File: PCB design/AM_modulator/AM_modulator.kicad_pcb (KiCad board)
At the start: 2 copper layers, 64.3 x 95.7 mm, 11 parts, among them Q1 MMBT3904

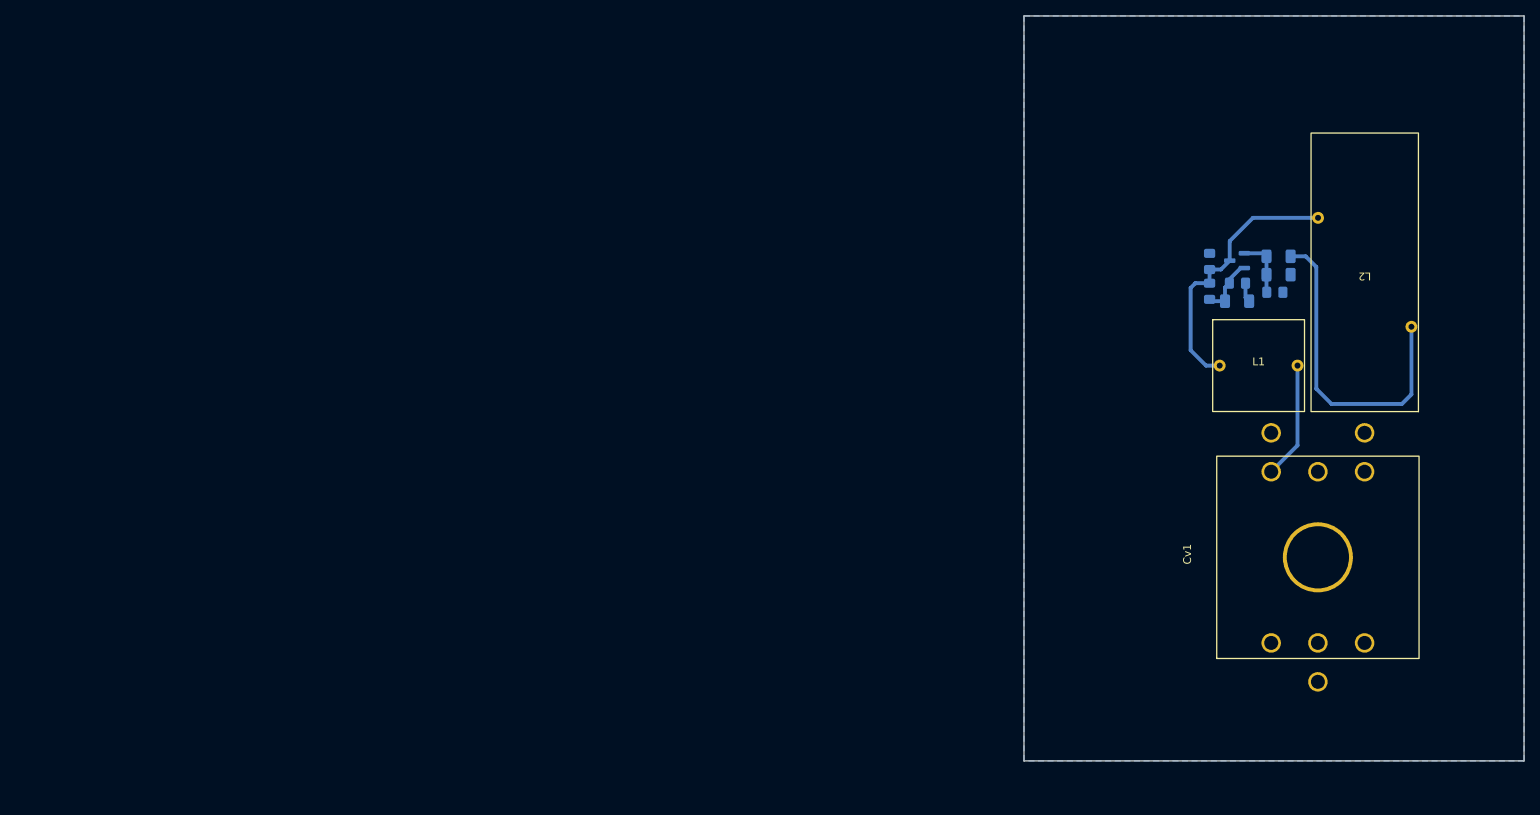
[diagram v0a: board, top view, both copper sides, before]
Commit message: Avances placa
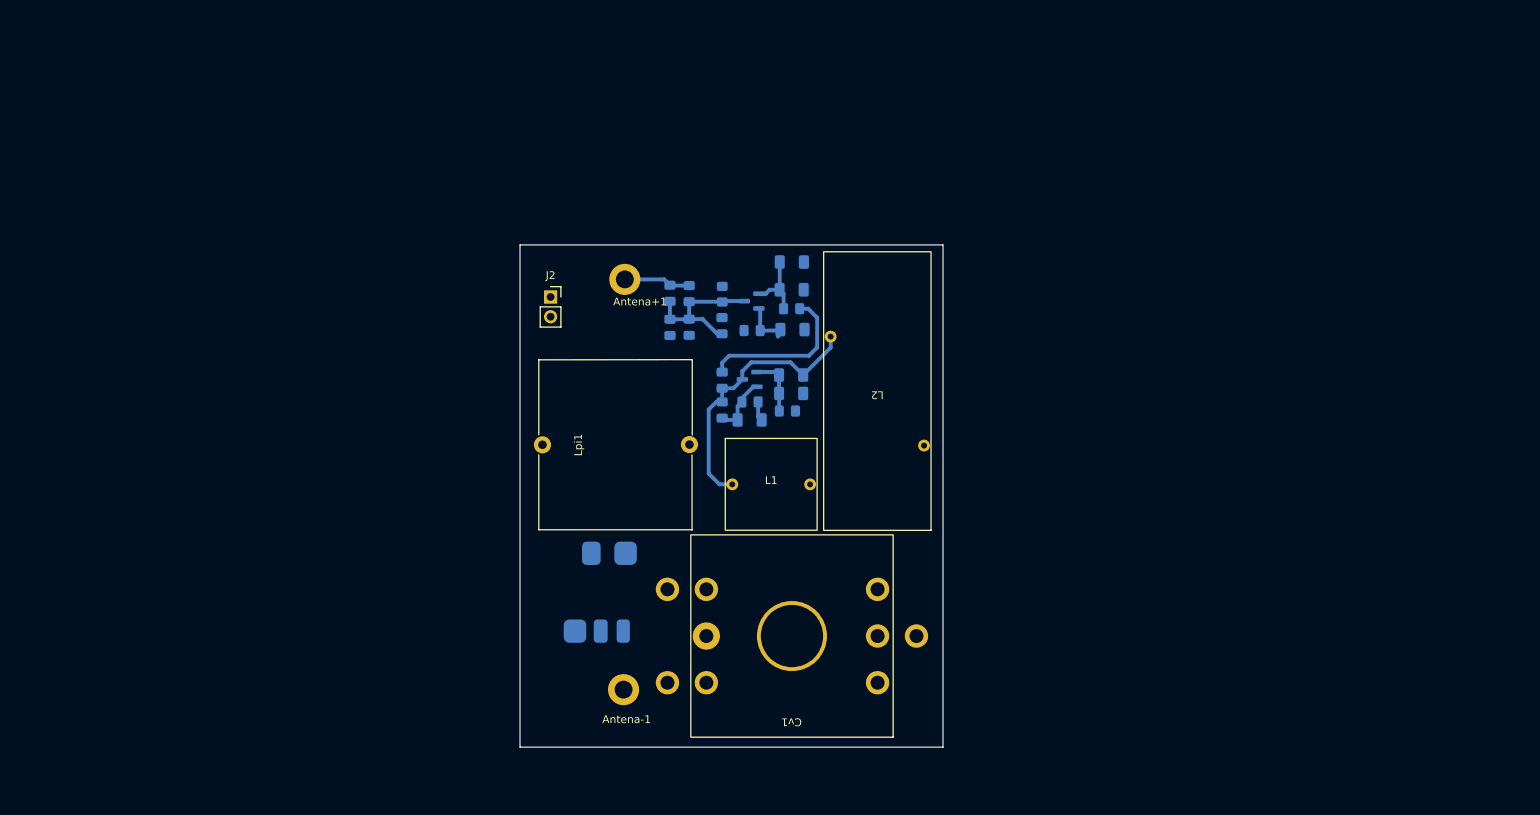
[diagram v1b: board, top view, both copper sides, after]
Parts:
- added Antena+1: Conn_01x01_Female, Connector_Pin:Pin_D1.4mm_L8.5mm_W2.8mm_FlatFork, F.Cu at (120.5, 63.7)
- added Antena-1: Conn_01x01_Female, Connector_Pin:Pin_D1.4mm_L8.5mm_W2.8mm_FlatFork, F.Cu at (120.3, 116.4)
- added CMLO1: 100n, Capacitor_SMD:C_0805_2012Metric_Pad1.18x1.45mm_HandSolder, B.Cu at (141.9, 67.5)
- added CMa1: 100n, Capacitor_SMD:C_0805_2012Metric_Pad1.18x1.45mm_HandSolder, B.Cu at (136.8, 70.3)
- added CMan1: 33p, Capacitor_SMD:C_0805_2012Metric_Pad1.18x1.45mm_HandSolder, B.Cu at (132.9, 69.7)
- added Cpi1: C, Capacitor_SMD:C_0805_2012Metric_Pad1.18x1.45mm_HandSolder, B.Cu at (128.7, 69.8)
- added Cpi11: C, Capacitor_SMD:C_0805_2012Metric_Pad1.18x1.45mm_HandSolder, B.Cu at (126.3, 69.9)
- added Cpi2: C, Capacitor_SMD:C_0805_2012Metric_Pad1.18x1.45mm_HandSolder, B.Cu at (128.7, 65.5)
- added Cpi21: C, Capacitor_SMD:C_0805_2012Metric_Pad1.18x1.45mm_HandSolder, B.Cu at (126.3, 65.5)
- added J1: AudioJack3, Jack Sigma:Jack_Sigma, B.Cu at (117.4, 103.9)
- added J2: Conn_01x02_Female, Connector_PinSocket_2.54mm:PinSocket_1x02_P2.54mm_Vertical, F.Cu at (110.9, 66.0)
- added Lpi1: L, Inductor_THT:L_Toroid_Vertical_L21.6mm_W9.1mm_P8.40mm_Bourns_5700, F.Cu at (109.9, 85.0)
- added QM1: MMBT3904, Package_TO_SOT_SMD:SOT-23, B.Cu at (136.8, 66.5)
- added RMb1: 100k, Resistor_SMD:R_1206_3216Metric_Pad1.30x1.75mm_HandSolder, B.Cu at (141.9, 65.0)
- added RMb2: 100k, Resistor_SMD:R_1206_3216Metric_Pad1.30x1.75mm_HandSolder, B.Cu at (141.9, 61.5)
- added RMc1: 220, Resistor_SMD:R_0805_2012Metric_Pad1.20x1.40mm_HandSolder, B.Cu at (133.0, 65.6)
- added RMe1: 100, Resistor_SMD:R_1206_3216Metric_Pad1.30x1.75mm_HandSolder, B.Cu at (142.0, 70.2)
- moved Cv1 68.3 mm to (141.9, 109.5), turned to 180 degrees
- moved C1 64.5 mm to (133.0, 80.5)
- moved C2 64.5 mm to (136.6, 79.4)
- moved C3 64.5 mm to (141.4, 80.6)
- moved C4 64.5 mm to (133.0, 76.7)
- moved L1 64.5 mm to (139.3, 90.0)
- moved L2 64.5 mm to (152.9, 78.0)
- moved Q1 64.5 mm to (136.5, 76.6)
- moved R1 64.5 mm to (141.8, 76.0)
- moved R2 64.5 mm to (141.8, 78.4)
- moved R3 64.5 mm to (136.5, 81.8)
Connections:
- C4 pad 2: /clapp_oscillator/Vout_30MHz_50Ohm -> /Mixer/LO
- L2 pad 1: +10V -> +12V
- R1 pad 1: +10V -> Net-(C1-Pad1)
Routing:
- net +10V: track 41.7 -> 0.00 mm
- net /Mixer/LO: track 0.00 -> 20.8 mm
- net /Antenna/RF_Antenna: track 0.00 -> 19.2 mm
- net Net-(Cv1-Pad1): track 15.0 -> 0.00 mm
- net Net-(CMLO1-Pad1): track 0.00 -> 9.09 mm
- net Net-(Antena+1-Pad1): track 0.00 -> 8.60 mm
- net Net-(CMa1-Pad1): track 0.00 -> 5.74 mm
- removed copper zone on B.Cu, net GND
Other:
- board size 64.3 x 95.7 mm -> 54.4 x 64.5 mm

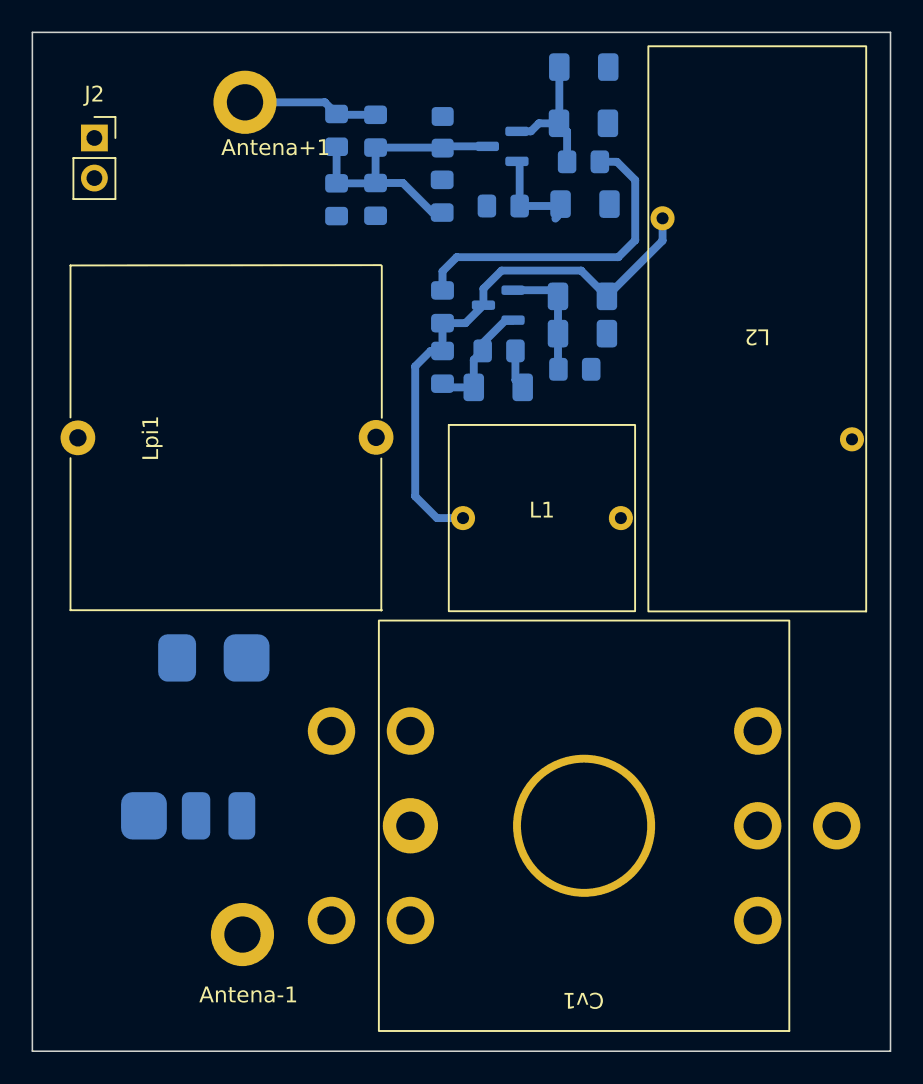
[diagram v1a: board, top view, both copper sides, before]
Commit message: Placa terminada
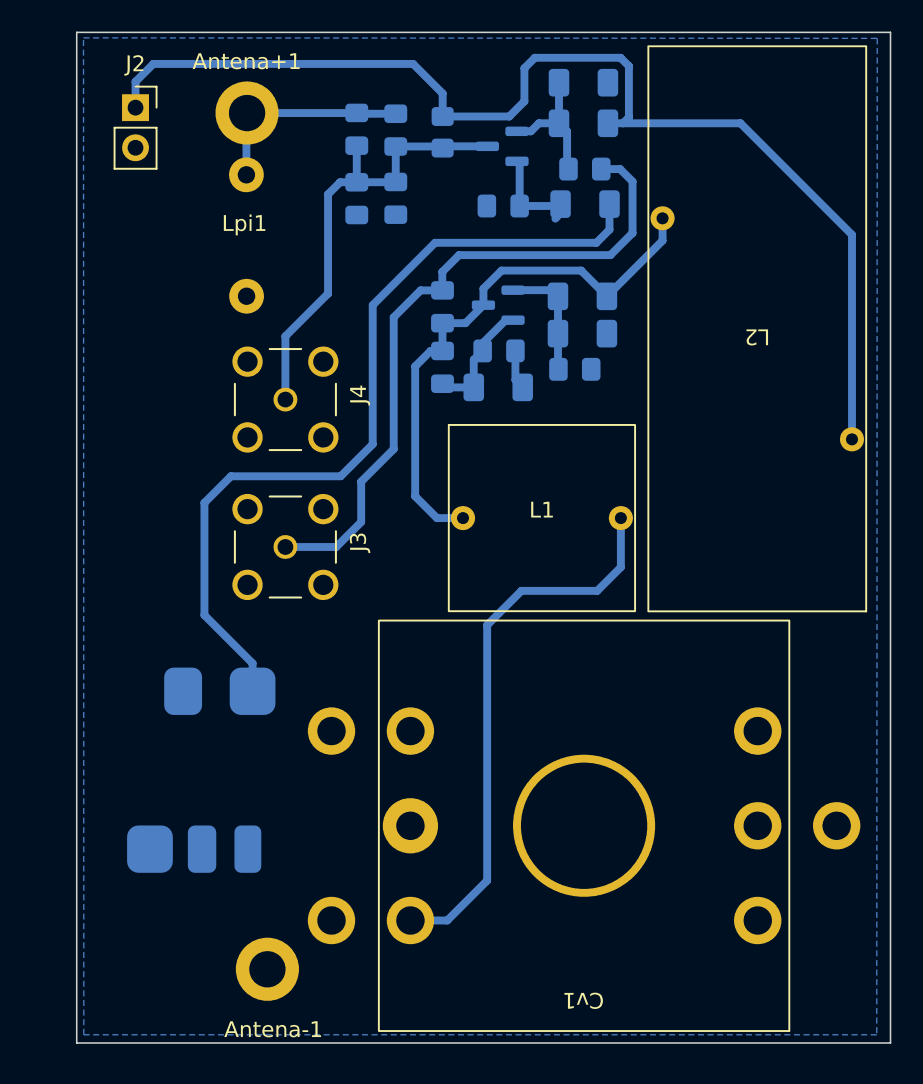
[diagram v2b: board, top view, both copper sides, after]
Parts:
- removed CMan1: 33p, Capacitor_SMD:C_0805_2012Metric_Pad1.18x1.45mm_HandSolder
- added J3: SMA_CONNECTOR, SMA_T:LPRS_SMA_CONNECTOR, F.Cu at (123.0, 91.9)
- added J4: SMA_CONNECTOR, SMA_T:LPRS_SMA_CONNECTOR, F.Cu at (123.0, 82.5)
- moved Lpi1 16.6 mm to (120.4, 72.1), turned to 0 degrees
- moved J2 3.24 mm to (113.5, 64.0)
- moved Antena-1 2.71 mm to (121.9, 118.6)
- moved J1 2.14 mm to (117.8, 106.0)
- moved Cpi11 1.28 mm to (127.5, 69.8)
- moved Cpi21 1.28 mm to (127.5, 65.4)
- moved Cpi1 1.28 mm to (130.0, 69.8)
- moved Cpi2 1.28 mm to (130.0, 65.5)
- moved RMb2 0.99 mm to (141.9, 62.5)
- moved Antena+1 0.69 mm to (120.6, 64.4)
- moved CMLO1 0.47 mm to (142.0, 67.9)
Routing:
- net +12V: track 0.00 -> 74.2 mm
- net /Mixer/Audio: track 0.00 -> 52.8 mm
- net Net-(Cv1-Pad1): track 0.00 -> 35.2 mm
- net /Mixer/LO: track 20.8 -> 42.9 mm
- net /Antenna/RF_Antenna: track 19.2 -> 29.2 mm
- net Net-(Antena+1-Pad1): track 8.60 -> 13.7 mm
- net Net-(CMLO1-Pad1): track 9.09 -> 8.12 mm
- added copper zone on B.Cu, net GND
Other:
- board size 54.4 x 64.5 mm -> 51.5 x 64 mm

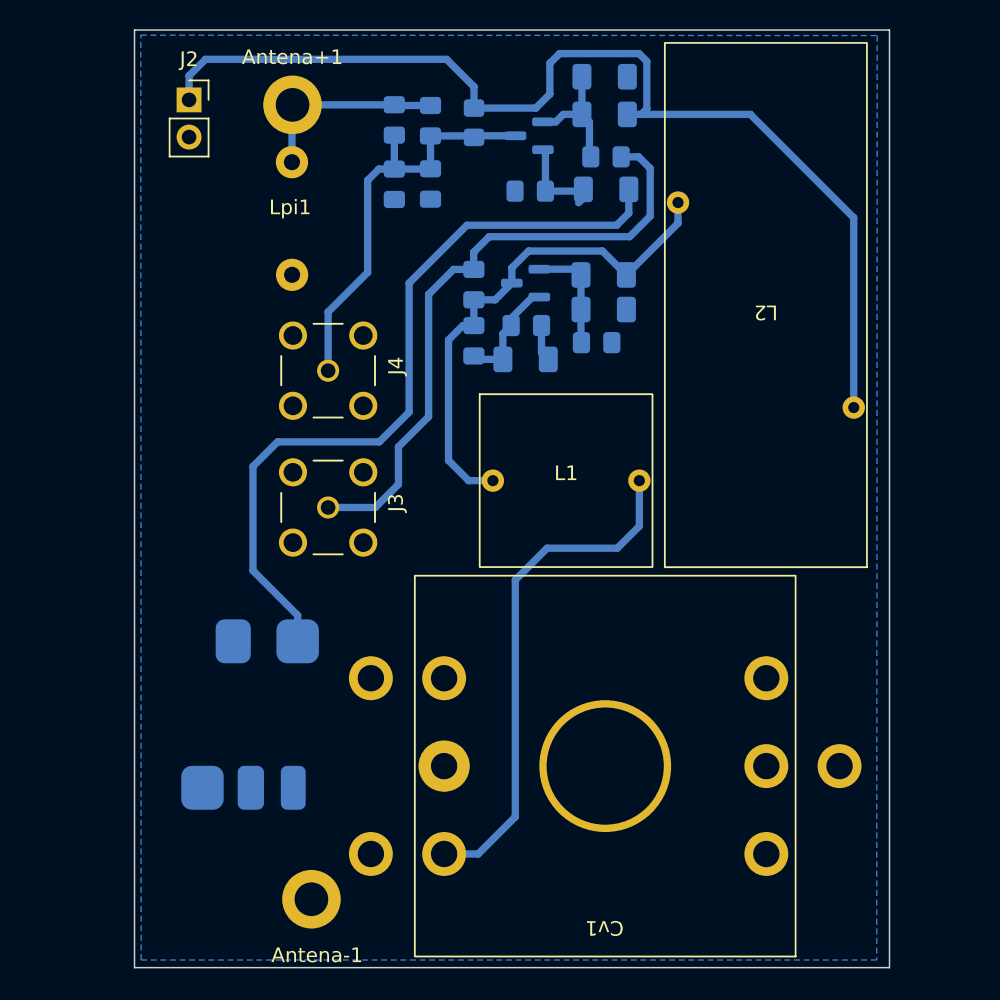
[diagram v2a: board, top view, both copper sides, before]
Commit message: PCB 2.0
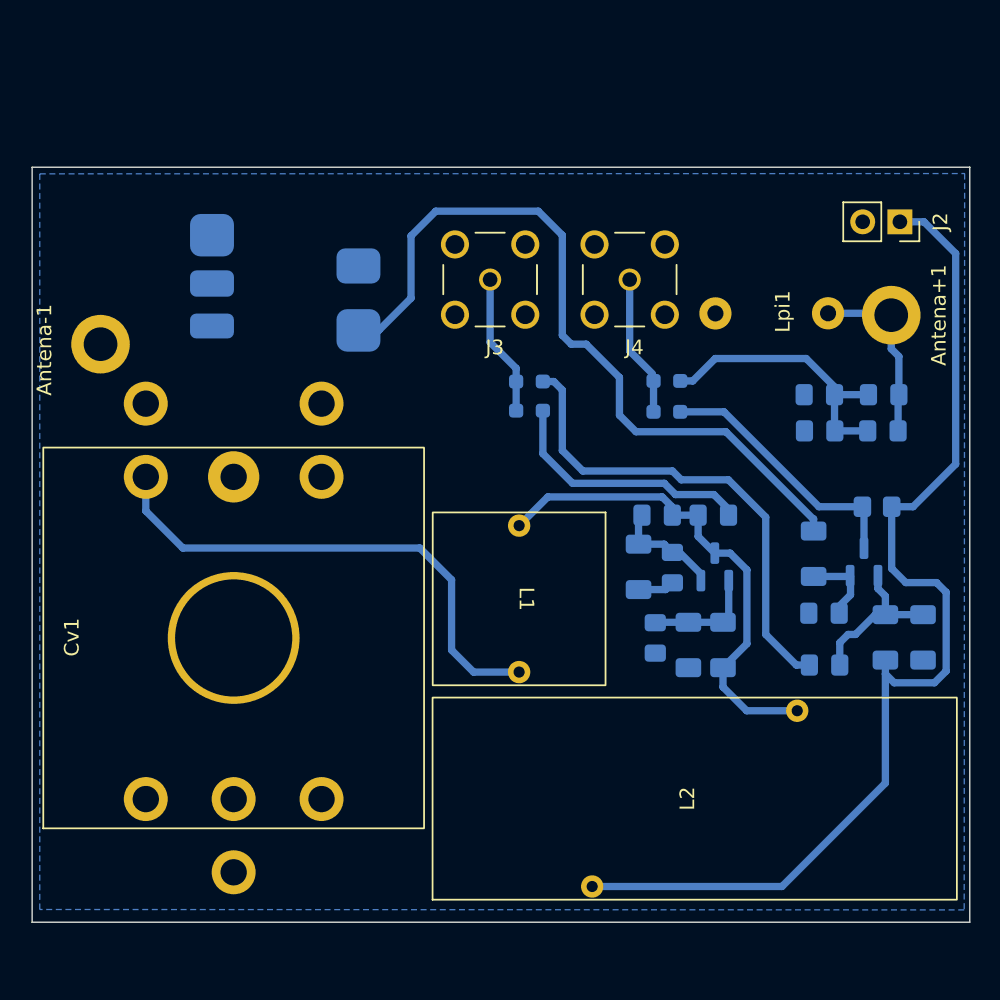
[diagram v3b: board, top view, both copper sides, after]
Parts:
- added SW1: SW_DIP_x01, Resistor_SMD:R_0603_1608Metric_Pad0.98x0.95mm_HandSolder, B.Cu at (136.8, 83.3)
- added SW2: SW_DIP_x01, Resistor_SMD:R_0603_1608Metric_Pad0.98x0.95mm_HandSolder, B.Cu at (146.2, 83.2)
- added SW3: SW_DIP_x01, Resistor_SMD:R_0603_1608Metric_Pad0.98x0.95mm_HandSolder, B.Cu at (136.8, 85.3)
- added SW4: SW_DIP_x01, Resistor_SMD:R_0603_1608Metric_Pad0.98x0.95mm_HandSolder, B.Cu at (146.2, 85.3)
- moved J2 49.2 mm to (162.1, 72.4), turned to -90 degrees
- moved RMb2 44.0 mm to (163.6, 100.7), turned to -90 degrees
- moved Antena+1 43.3 mm to (161.5, 78.7), turned to -90 degrees
- moved Antena-1 40.5 mm to (107.5, 80.7), turned to -90 degrees
- moved RMb1 40.5 mm to (161.1, 100.7), turned to 90 degrees
- moved Cpi21 38.3 mm to (161.0, 84.2), turned to 0 degrees
- moved RMc1 38.0 mm to (160.5, 91.8), turned to 180 degrees
- moved CMLO1 37.8 mm to (156.9, 102.6), turned to 180 degrees
- moved Cpi2 37.5 mm to (160.9, 86.6), turned to 0 degrees
- moved QM1 37.0 mm to (159.6, 95.6), turned to 90 degrees
- moved CMa1 35.1 mm to (156.9, 99.1)
- moved L2 34.0 mm to (148.1, 111.8), turned to 90 degrees
- moved Lpi1 33.6 mm to (153.3, 78.4), turned to -90 degrees
- moved Cpi11 32.4 mm to (156.6, 84.2), turned to 0 degrees
- moved Cpi1 31.5 mm to (156.6, 86.6), turned to 180 degrees
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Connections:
- C4 pad 2: /Mixer/LO -> Net-(C4-Pad2)
- J3 pad 1: /Mixer/LO -> /clapp_oscillator/Vout_30MHz_50Ohm
- J4 pad 1: /Antenna/RF_Antenna -> /Mixer/RF
- QM1 pad 3: /Antenna/RF_Antenna -> Net-(QM1-Pad3)
- RMc1 pad 2: /Antenna/RF_Antenna -> Net-(QM1-Pad3)
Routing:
- net Net-(QM1-Pad3): track 0.00 -> 18.1 mm
- net Net-(C4-Pad2): track 0.00 -> 17.6 mm
- net /clapp_oscillator/Vout_30MHz_50Ohm: track 0.00 -> 9.69 mm
- net /Antenna/RF_Antenna: track 29.2 -> 19.5 mm
- net /Mixer/LO: track 42.9 -> 33.3 mm
- net /Mixer/RF: track 0.00 -> 9.19 mm
- net Net-(CMLO1-Pad1): track 8.12 -> 11.2 mm
- net Net-(C1-Pad1): track 35.2 -> 34.0 mm
- net +12V: track 74.2 -> 75.2 mm
- net /Mixer/Audio: track 52.8 -> 52.0 mm
- net Net-(Antena+1-Pad1): track 13.7 -> 12.9 mm
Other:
- board size 51.5 x 64 mm -> 64 x 51.5 mm
